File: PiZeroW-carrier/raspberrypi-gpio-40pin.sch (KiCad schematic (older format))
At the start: 8 parts, among them J1 PI40HAT, J2 CONN_02X02

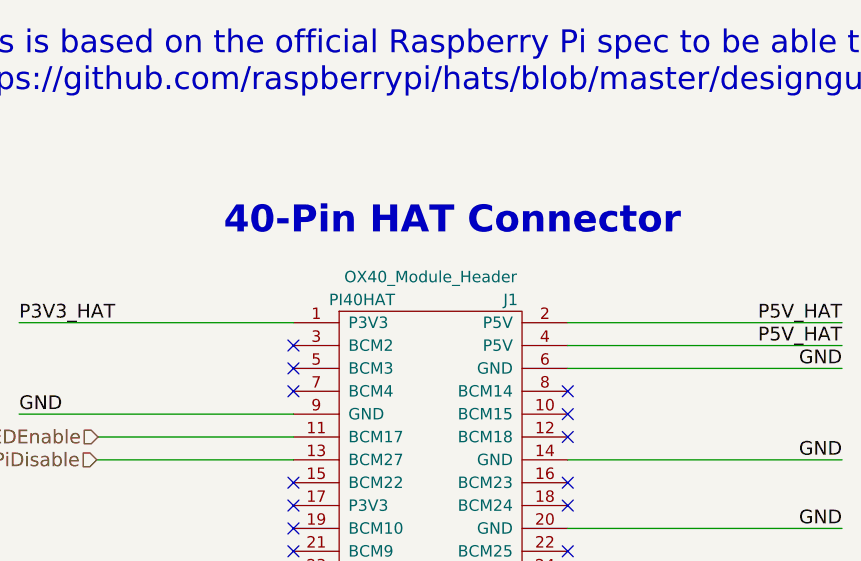
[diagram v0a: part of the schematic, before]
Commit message: netlist update and read into pcb
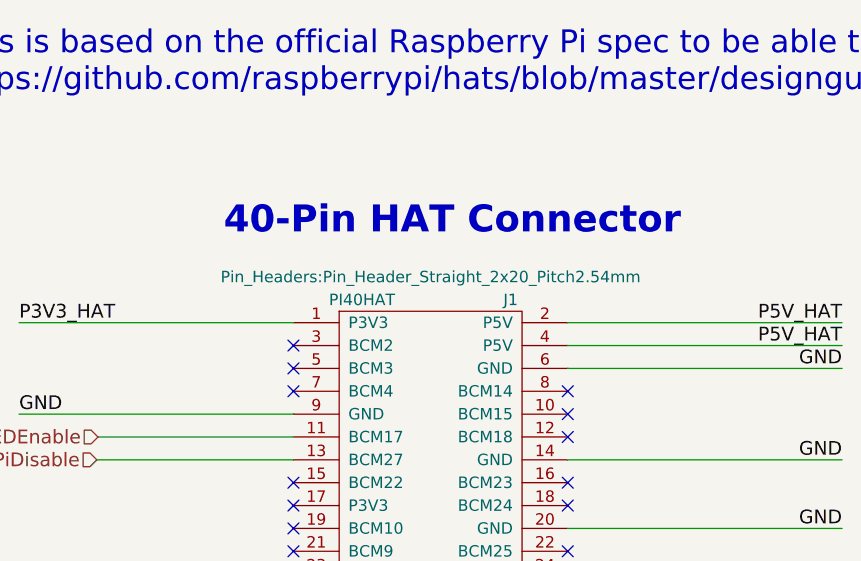
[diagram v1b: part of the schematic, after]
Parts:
- J1: footprint OX40_Module_Header -> Pin_Headers:Pin_Header_Straight_2x20_Pitch2.54mm
- J2: footprint Pin_Headers:Pin_Header_Straight_2x02 -> Pin_Headers:Pin_Header_Straight_2x02_Pitch2.54mm
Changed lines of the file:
@@
 EESchema Schematic File Version 2
+LIBS:PiZeroW-carrier-rescue
 LIBS:power
 LIBS:device
@@
 F 0 "J2" H 6100 4800 50  0000 C CNN
 F 1 "CONN_02X02" H 6100 4500 50  0000 C CNN
-F 2 "Pin_Headers:Pin_Header_Straight_2x02" H 6100 3450 50  0001 C CNN
+F 2 "Pin_Headers:Pin_Header_Straight_2x02_Pitch2.54mm" H 6100 3450 50  0001 C CNN
 F 3 "" H 6100 3450 50  0000 C CNN
 	1    6100 4650
@@
 F 0 "J1" H 3300 2350 50  0000 C CNN
 F 1 "PI40HAT" H 2650 2350 50  0000 C CNN
-F 2 "OX40_Module_Header" H 2950 2450 50  0000 C CNN
+F 2 "Pin_Headers:Pin_Header_Straight_2x20_Pitch2.54mm" H 2950 2450 50  0000 C CNN
 F 3 "" H 2250 2250 50  0000 C CNN
 	1    2950 2250
